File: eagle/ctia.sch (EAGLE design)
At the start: 16 parts, among them IC1 IVC102UADAPTOR, IC2 LT1352PA, IC3 AD580H

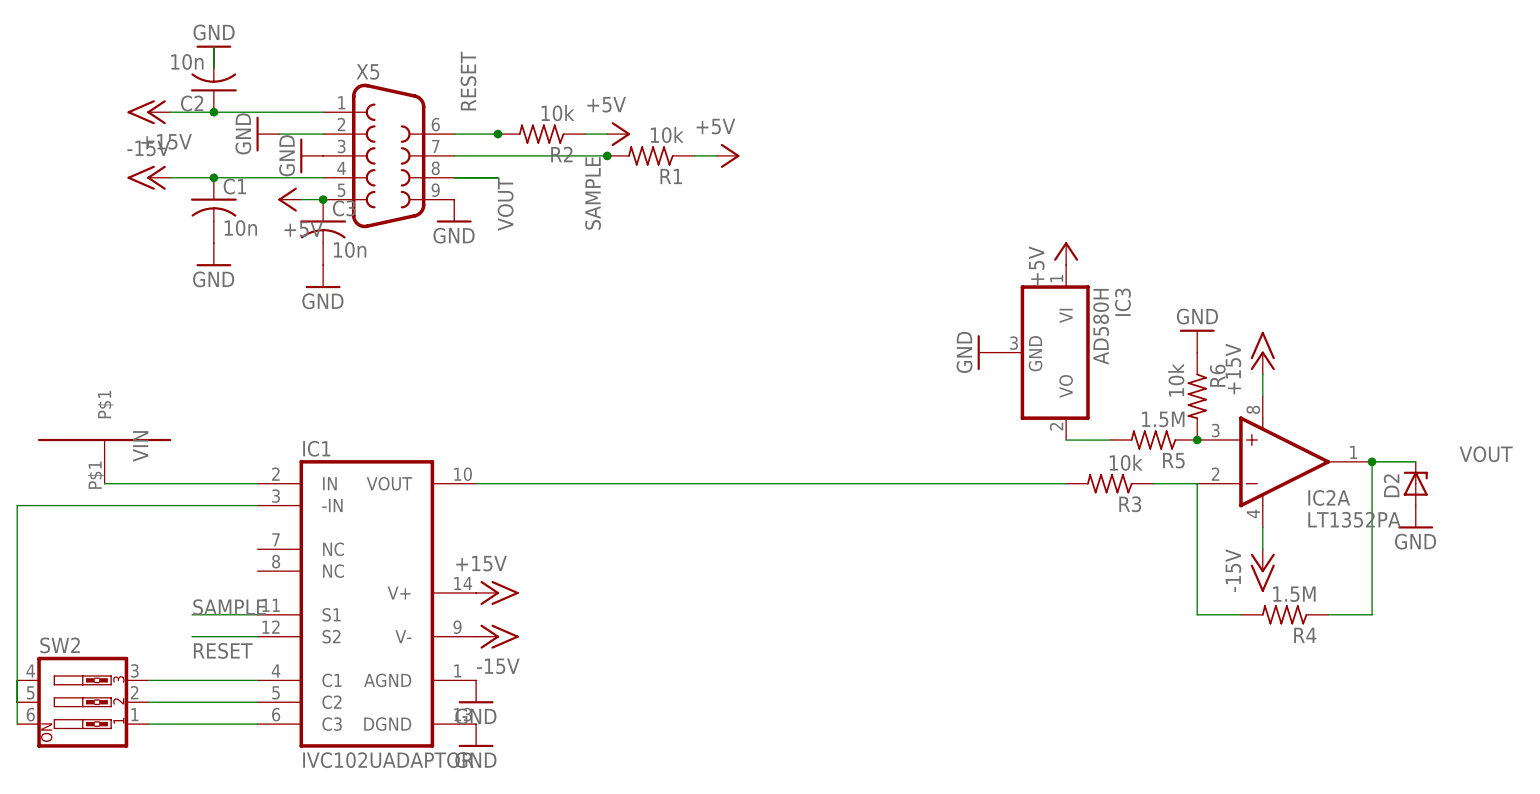
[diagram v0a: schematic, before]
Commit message: lower noise
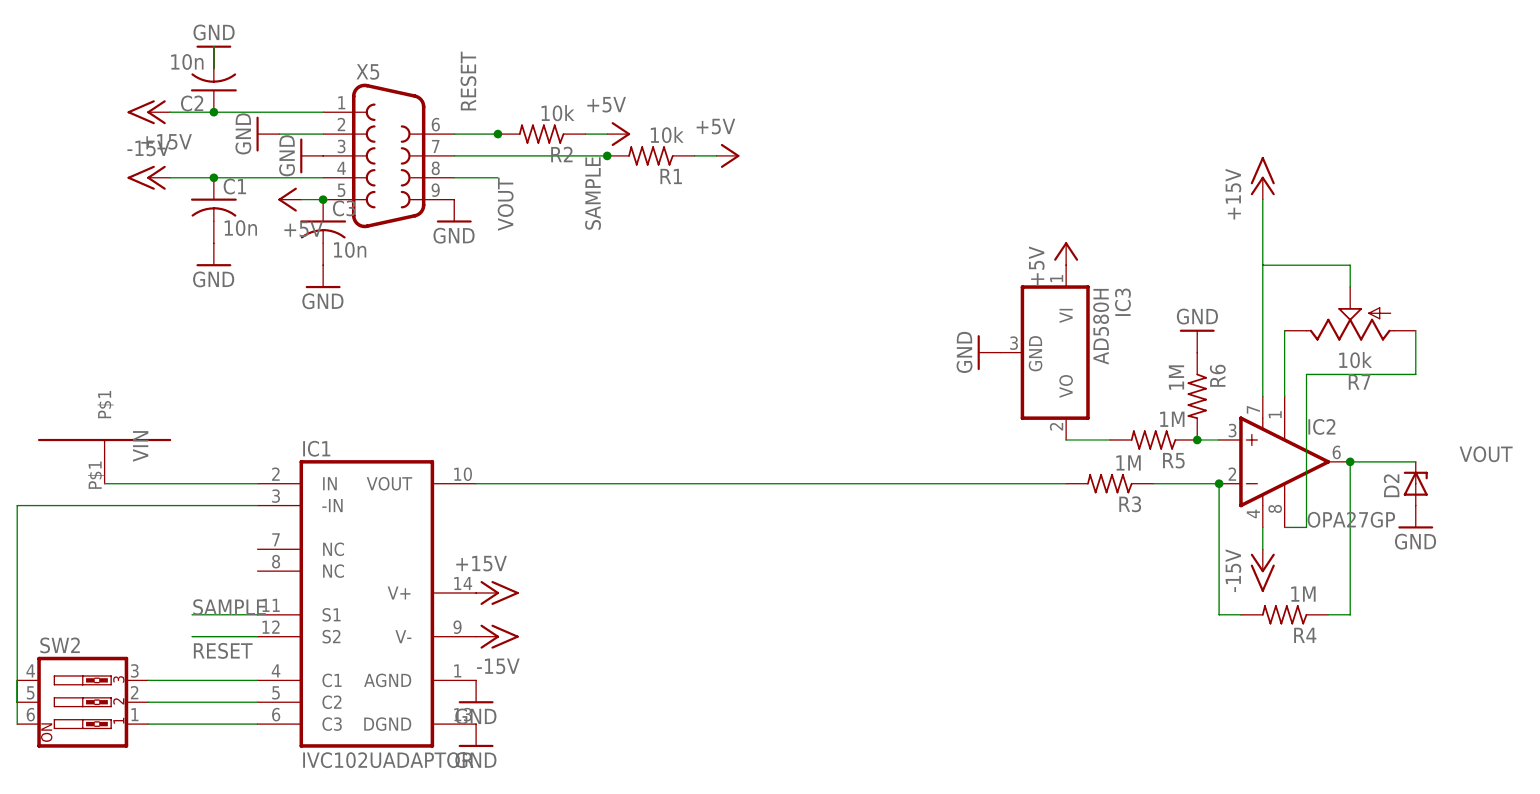
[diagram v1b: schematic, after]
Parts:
- added R7: 10k, pot:TRIM_US-B64Y
- IC2: value LT1352PA -> OPA27GP; device linear-technology:LT1352PA -> linear:OPA27GP
- R3, R6: value 10k -> 1M
- R4, R5: value 1.5M -> 1M
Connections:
- new net N$10: IC2.OFF2, R7.A
- new net N$9: IC2.OFF1, R7.E
- net +15V: now also IC2.V+, R7.S; no longer IC2A.V+
- net -15V: now also IC2.V-; no longer IC2A.V-
- net N$6: now also IC2.-IN; no longer IC2A.-IN
- net N$7: now also IC2.+IN; no longer IC2A.+IN
- net VOUT: now also IC2.OUT; no longer IC2A.OUT
